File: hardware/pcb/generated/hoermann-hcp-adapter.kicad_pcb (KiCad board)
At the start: 2 copper layers, 65 x 44.5 mm, 6 parts, among them J1 HCP2 6P6C, U1 ESP32-C3 Super Mini, U2 Isolated RS485

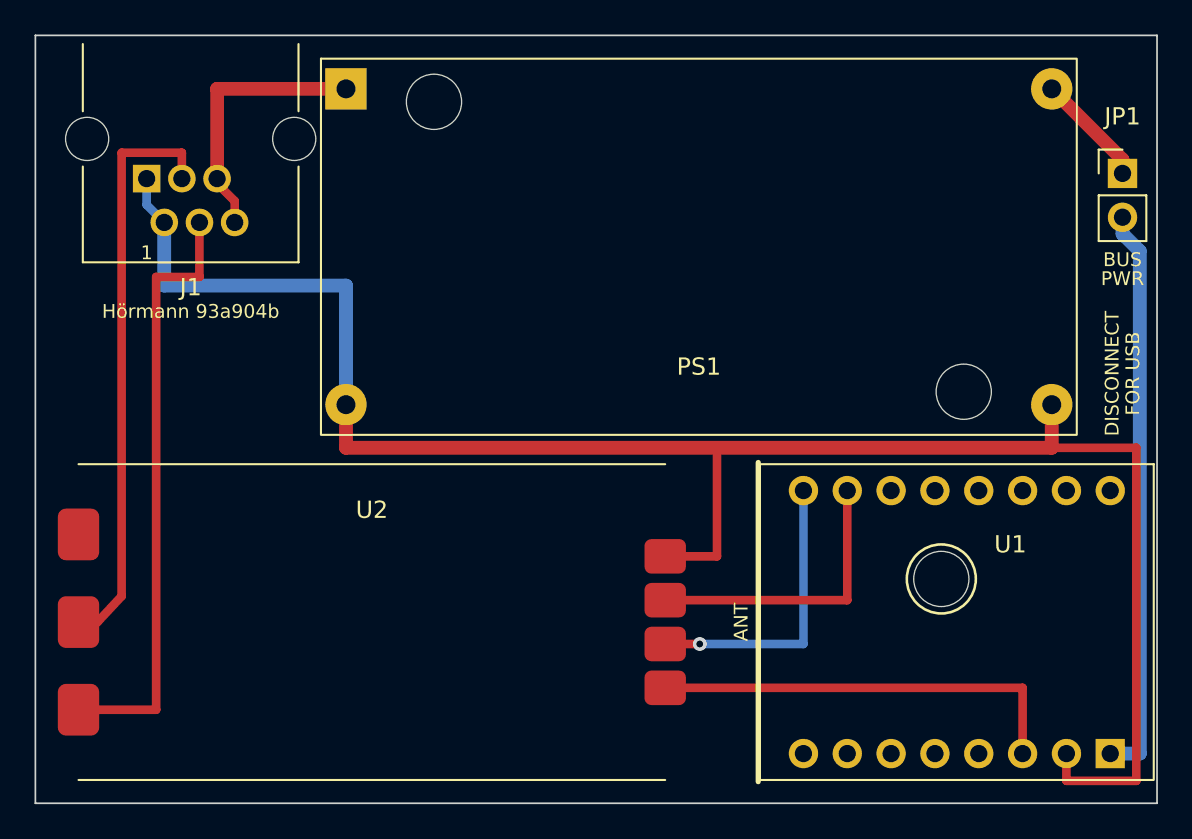
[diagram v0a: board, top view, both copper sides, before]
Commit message: Regenerate outputs
Co-Authored-By: Claude Fable 5.1 <noreply@anthropic.com>
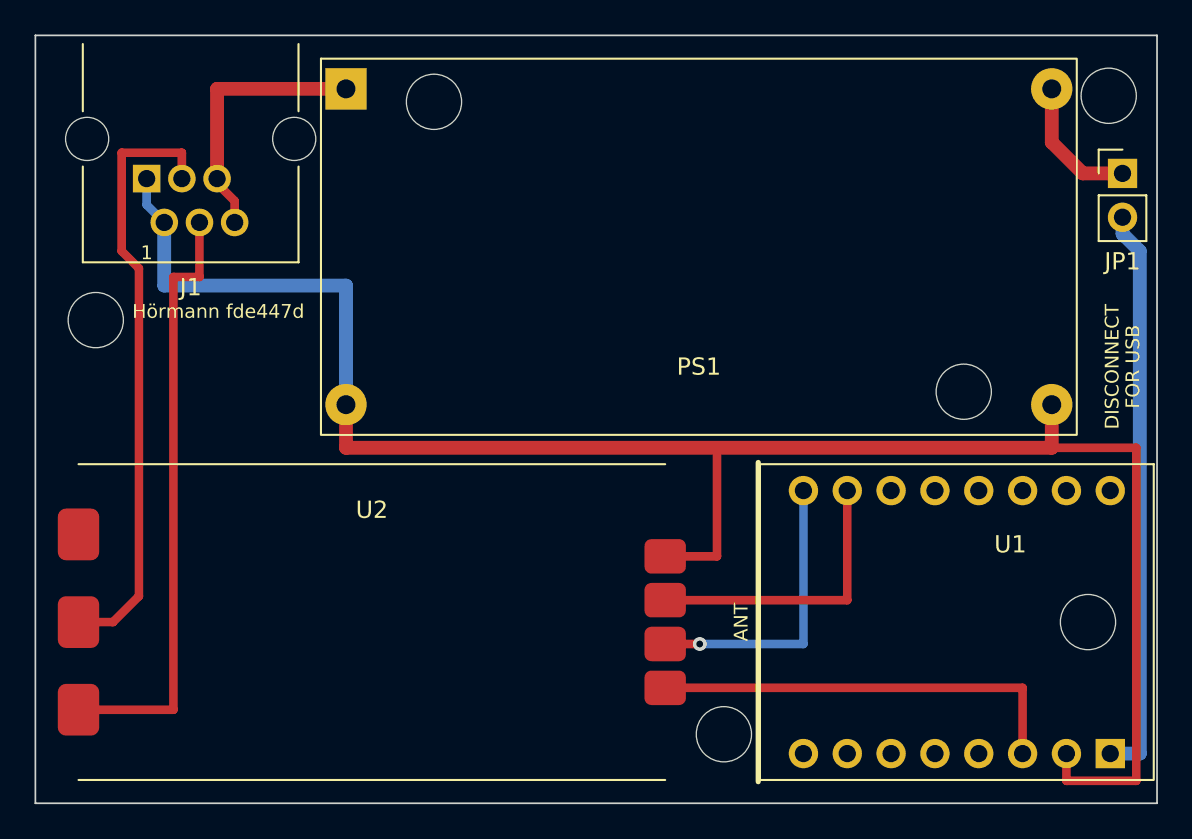
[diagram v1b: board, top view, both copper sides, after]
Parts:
- added H2: M3, HCP:MountingHole_3.2mm_NoCourtyard, F.Cu at (178.2, 71.5)
- added H3: M3, HCP:MountingHole_3.2mm_NoCourtyard, F.Cu at (155.9, 108.5)
- added H4: M3, HCP:MountingHole_3.2mm_NoCourtyard, F.Cu at (177.0, 102.0)
- moved H1 51.2 mm to (119.5, 84.5)
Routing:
- net HCP_B_MINUS: track 33.8 -> 35.2 mm
- net BUCK_5V: track 6.60 -> 7.95 mm
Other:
- board text added: "Hörmann HCP2 Adapter fde447d"
- board text added: "Hörmann fde447d"
- board text removed: "BUS"
- board text removed: "Hörmann 93a904b"
- board text removed: "Hörmann HCP2 Adapter 93a904b"
- board text removed: "PWR"
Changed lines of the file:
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@@
   	(tags "Through hole pin header THT 1x02 2.54mm single row")
   	(property "Reference" "JP1"
-  		(at 0.00 -3.30 0)
+  		(at 0.00 5.10 0)
   		(layer "F.SilkS")
   		(effects
@@
   (footprint "HCP:MountingHole_3.2mm_NoCourtyard"
     (layer "F.Cu")
-    (at 168.5 99.5 0)
+    (at 119.5 84.5 0)
     (descr "M3 mounting hole without courtyard, for placement under socketed modules")
     (tags "mounting hole M3")
@@
     (property "Description" "" (at 0 0 0) (layer "F.Fab") (hide yes) (effects (font (size 1.0 1.0) (thickness 0.15))))
     (attr exclude_from_pos_files exclude_from_bom)
-    (fp_circle (center 0 0) (end 2.0 0) (stroke (width 0.15) (type default)) (fill none) (layer "F.SilkS"))
+    (pad "" np_thru_hole circle (at 0 0) (size 3.2 3.2) (drill 3.2) (layers "*.Cu" "*.Mask"))
+    (embedded_fonts no)
+  )
+  (footprint "HCP:MountingHole_3.2mm_NoCourtyard"
+    (layer "F.Cu")
+    (at 178.2 71.5 0)
+    (descr "M3 mounting hole without courtyard, for placement under socketed modules")
+    (tags "mounting hole M3")
+    (property "Reference" "H2" (at 0 -3 0) (layer "F.SilkS") (hide yes) (effects (font (size 1.0 1.0) (thickness 0.15))))
+    (property "Value" "M3" (at 0 3 0) (layer "F.Fab") (hide yes) (effects (font (size 1.0 1.0) (thickness 0.15))))
+    (property "Datasheet" "" (at 0 0 0) (layer "F.Fab") (hide yes) (effects (font (size 1.0 1.0) (thickness 0.15))))
+    (property "Description" "" (at 0 0 0) (layer "F.Fab") (hide yes) (effects (font (size 1.0 1.0) (thickness 0.15))))
+    (attr exclude_from_pos_files exclude_from_bom)
+    (pad "" np_thru_hole circle (at 0 0) (size 3.2 3.2) (drill 3.2) (layers "*.Cu" "*.Mask"))
+    (embedded_fonts no)
+  )
+  (footprint "HCP:MountingHole_3.2mm_NoCourtyard"
+    (layer "F.Cu")
+    (at 155.9 108.5 0)
+    (descr "M3 mounting hole without courtyard, for placement under socketed modules")
+    (tags "mounting hole M3")
+    (property "Reference" "H3" (at 0 -3 0) (layer "F.SilkS") (hide yes) (effects (font (size 1.0 1.0) (thickness 0.15))))
+    (property "Value" "M3" (at 0 3 0) (layer "F.Fab") (hide yes) (effects (font (size 1.0 1.0) (thickness 0.15))))
+    (property "Datasheet" "" (at 0 0 0) (layer "F.Fab") (hide yes) (effects (font (size 1.0 1.0) (thickness 0.15))))
+    (property "Description" "" (at 0 0 0) (layer "F.Fab") (hide yes) (effects (font (size 1.0 1.0) (thickness 0.15))))
+    (attr exclude_from_pos_files exclude_from_bom)
+    (pad "" np_thru_hole circle (at 0 0) (size 3.2 3.2) (drill 3.2) (layers "*.Cu" "*.Mask"))
+    (embedded_fonts no)
+  )
+  (footprint "HCP:MountingHole_3.2mm_NoCourtyard"
+    (layer "F.Cu")
+    (at 177.0 102.0 0)
+    (descr "M3 mounting hole without courtyard, for placement under socketed modules")
+    (tags "mounting hole M3")
+    (property "Reference" "H4" (at 0 -3 0) (layer "F.SilkS") (hide yes) (effects (font (size 1.0 1.0) (thickness 0.15))))
+    (property "Value" "M3" (at 0 3 0) (layer "F.Fab") (hide yes) (effects (font (size 1.0 1.0) (thickness 0.15))))
+    (property "Datasheet" "" (at 0 0 0) (layer "F.Fab") (hide yes) (effects (font (size 1.0 1.0) (thickness 0.15))))
+    (property "Description" "" (at 0 0 0) (layer "F.Fab") (hide yes) (effects (font (size 1.0 1.0) (thickness 0.15))))
+    (attr exclude_from_pos_files exclude_from_bom)
     (pad "" np_thru_hole circle (at 0 0) (size 3.2 3.2) (drill 3.2) (layers "*.Cu" "*.Mask"))
     (embedded_fonts no)
@@
   (segment (start 155.5 91.9) (end 155.5 98.19) (width 0.5) (layer "F.Cu") (net 1))
   (segment (start 155.5 98.19) (end 152.5 98.19) (width 0.5) (layer "F.Cu") (net 1))
-  (segment (start 174.9 71.1) (end 179.0 75.2) (width 0.8) (layer "F.Cu") (net 5))
-  (segment (start 179.0 75.2) (end 179.0 76.0) (width 0.8) (layer "F.Cu") (net 5))
+  (segment (start 174.9 71.1) (end 174.9 74.2) (width 0.8) (layer "F.Cu") (net 5))
+  (segment (start 174.9 74.2) (end 176.7 76.0) (width 0.8) (layer "F.Cu") (net 5))
+  (segment (start 176.7 76.0) (end 179.0 76.0) (width 0.8) (layer "F.Cu") (net 5))
   (segment (start 179.0 78.54) (end 179.0 79.5) (width 0.8) (layer "B.Cu") (net 6))
   (segment (start 179.0 79.5) (end 180.0 80.5) (width 0.8) (layer "B.Cu") (net 6))
@@
   (segment (start 124.49 76.3) (end 124.49 74.8) (width 0.5) (layer "F.Cu") (net 4))
   (segment (start 124.49 74.8) (end 121.0 74.8) (width 0.5) (layer "F.Cu") (net 4))
-  (segment (start 121.0 74.8) (end 121.0 100.5) (width 0.5) (layer "F.Cu") (net 4))
-  (segment (start 121.0 100.5) (end 119.6 102.0) (width 0.5) (layer "F.Cu") (net 4))
-  (segment (start 119.6 102.0) (end 118.5 102.0) (width 0.5) (layer "F.Cu") (net 4))
+  (segment (start 121.0 74.8) (end 121.0 80.5) (width 0.5) (layer "F.Cu") (net 4))
+  (segment (start 121.0 80.5) (end 122.0 81.5) (width 0.5) (layer "F.Cu") (net 4))
+  (segment (start 122.0 81.5) (end 122.0 100.5) (width 0.5) (layer "F.Cu") (net 4))
+  (segment (start 122.0 100.5) (end 120.5 102.0) (width 0.5) (layer "F.Cu") (net 4))
+  (segment (start 120.5 102.0) (end 118.5 102.0) (width 0.5) (layer "F.Cu") (net 4))
   (segment (start 125.51 78.84) (end 125.51 82.0) (width 0.5) (layer "F.Cu") (net 3))
-  (segment (start 125.51 82.0) (end 123.0 82.0) (width 0.5) (layer "F.Cu") (net 3))
-  (segment (start 123.0 82.0) (end 123.0 107.08) (width 0.5) (layer "F.Cu") (net 3))
-  (segment (start 123.0 107.08) (end 118.5 107.08) (width 0.5) (layer "F.Cu") (net 3))
+  (segment (start 125.51 82.0) (end 124.0 82.0) (width 0.5) (layer "F.Cu") (net 3))
+  (segment (start 124.0 82.0) (end 124.0 107.08) (width 0.5) (layer "F.Cu") (net 3))
+  (segment (start 124.0 107.08) (end 118.5 107.08) (width 0.5) (layer "F.Cu") (net 3))
   (via (at 154.5 103.27) (size 0.8) (drill 0.4) (layers "F.Cu" "B.Cu") (net 8))
   (gr_rect (start 116.0 68.0) (end 181.0 112.5) (stroke (width 0.1) (type default)) (fill none) (layer "Edge.Cuts"))
-  (gr_text "Hörmann 93a904b" (at 125.0 84.0 0) (layer "F.SilkS") (effects (font (size 0.8 0.8) (thickness 0.15))))
+  (gr_text "Hörmann fde447d" (at 126.6 84.0 0) (layer "F.SilkS") (effects (font (size 0.8 0.8) (thickness 0.15))))
   (gr_text "1" (at 122.45 80.6 0) (layer "F.SilkS") (effects (font (size 0.8 0.8) (thickness 0.15))))
-  (gr_text "BUS" (at 179.0 81.0 0) (layer "F.SilkS") (effects (font (size 0.8 0.8) (thickness 0.15))))
-  (gr_text "PWR" (at 179.0 82.1 0) (layer "F.SilkS") (effects (font (size 0.8 0.8) (thickness 0.15))))
-  (gr_text "DISCONNECT" (at 178.4 87.6 90) (layer "F.SilkS") (effects (font (size 0.8 0.8) (thickness 0.15))))
-  (gr_text "FOR USB" (at 179.6 87.6 90) (layer "F.SilkS") (effects (font (size 0.8 0.8) (thickness 0.15))))
+  (gr_text "DISCONNECT" (at 178.4 87.2 90) (layer "F.SilkS") (effects (font (size 0.8 0.8) (thickness 0.15))))
+  (gr_text "FOR USB" (at 179.6 87.2 90) (layer "F.SilkS") (effects (font (size 0.8 0.8) (thickness 0.15))))
   (gr_text "ANT" (at 156.9 102.0 90) (layer "F.SilkS") (effects (font (size 0.8 0.8) (thickness 0.15))))
-  (gr_text "Hörmann HCP2 Adapter 93a904b" (at 141.0 98.5 0) (layer "B.SilkS") (effects (font (size 1.5 1.5) (thickness 0.15)) (justify mirror)))
+  (gr_text "Hörmann HCP2 Adapter fde447d" (at 141.0 98.5 0) (layer "B.SilkS") (effects (font (size 1.5 1.5) (thickness 0.15)) (justify mirror)))
   (gr_text "(C) 2026 Thies Gerken" (at 141.0 101.5 0) (layer "B.SilkS") (effects (font (size 1.2 1.2) (thickness 0.15)) (justify mirror)))
   (embedded_fonts no)
